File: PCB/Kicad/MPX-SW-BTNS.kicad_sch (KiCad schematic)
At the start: 34 parts, among them SW13 SWCUEL, SW14 SWPLAYL, SW15 SWRANGEL, SW16 SWSYNCL, SW17 SWLOOPL, SW18 SWSHIFTL, SW19 SWSHIFTR, SW20 SWPCUEL1, SW21 SWPCUEL2, SW22 SWCUER, SW23 SWPLAYR, SW24 SWRANGER, SW25 SWLOOPR, SW26 SWPCUEL3, SW27 SWSYNCR, SW28 SWDECKSEL, SW29 SWPADL5, SW30 SWPADL1, SW31 SWPADL6, SW32 SWPADL2, SW33 SWPADL7, SW34 SWPADL3, SW35 SWPADL4, SW36 SWPADL8, SW37 SWPADR5, SW38 SWPADR1, SW39 SWPADR6, SW40 SWPADR2, SW41 SWPADR7, SW42 SWPADR3, SW43 SWPADR4, SW44 SWPADR8

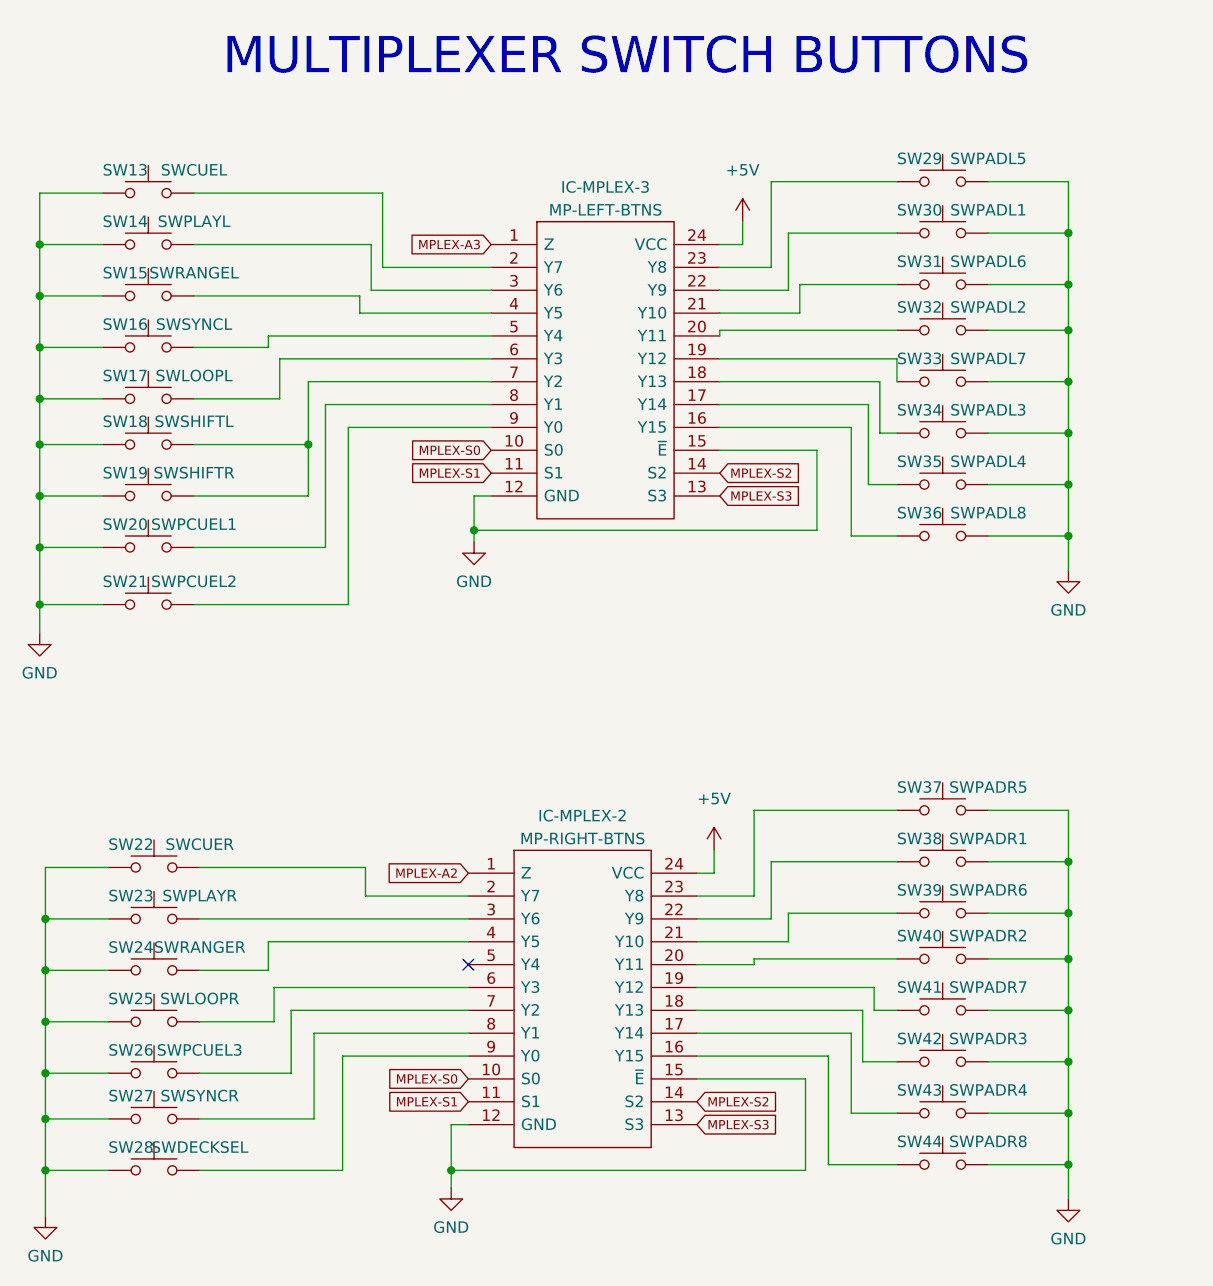
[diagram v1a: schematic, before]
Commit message: routing WIP
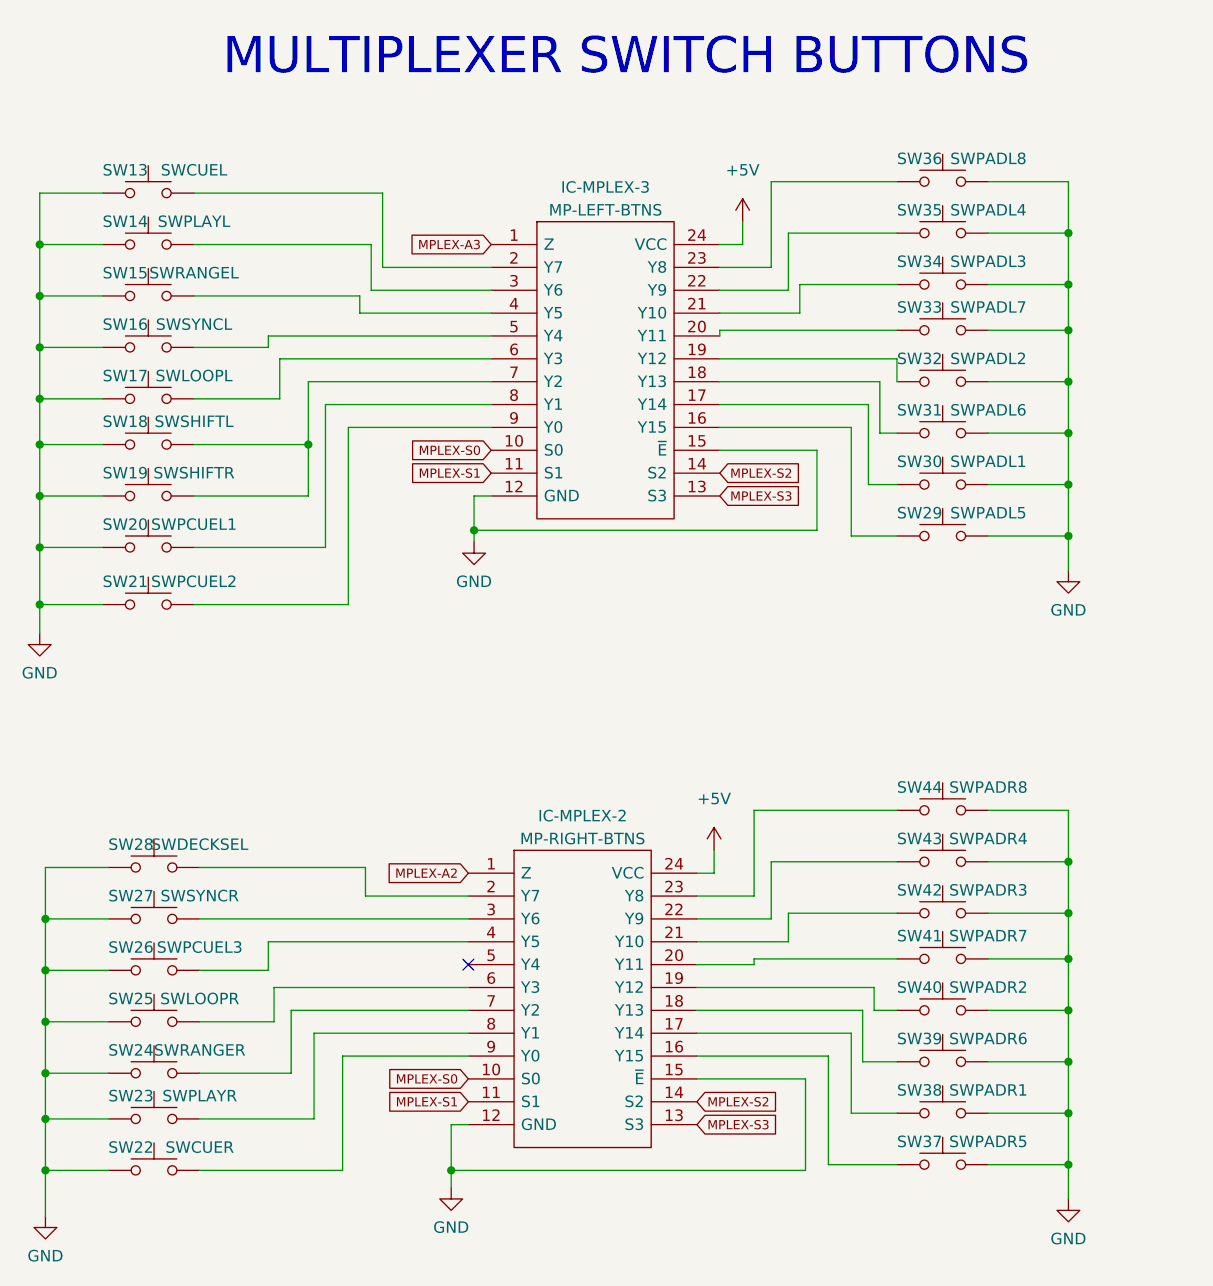
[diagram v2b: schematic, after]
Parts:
- SW13, SW14, SW15, SW16, SW17, SW18, SW19, SW20, SW21, SW22, SW23, SW24, SW25, SW26, SW27, SW28: footprint Library:SW_PUSH_6mm_H8mm -> Library:SW_Push_1P1T_NO_6x6mm_H8mm
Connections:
- net at SW41.1: now also IC-MPLEX-2.20 (Y11); no longer IC-MPLEX-2.19 (Y12)
- net at SW27.2: now also IC-MPLEX-2.3 (Y6); no longer IC-MPLEX-2.8 (Y1)
- net at IC-MPLEX-3.16 (Y15): now also SW29.1; no longer SW36.1
- net at IC-MPLEX-3.17 (Y14): now also SW30.1; no longer SW35.1
- net at IC-MPLEX-3.18 (Y13): now also SW31.1; no longer SW34.1
- net at IC-MPLEX-3.19 (Y12): now also SW32.1; no longer SW33.1
- net at IC-MPLEX-3.20 (Y11): now also SW33.1; no longer SW32.1
- net at IC-MPLEX-3.21 (Y10): now also SW34.1; no longer SW31.1
- net at IC-MPLEX-3.22 (Y9): now also SW35.1; no longer SW30.1
- net at IC-MPLEX-3.23 (Y8): now also SW36.1; no longer SW29.1
- net at SW40.1: now also IC-MPLEX-2.19 (Y12); no longer IC-MPLEX-2.20 (Y11)
- net at SW44.1: now also IC-MPLEX-2.23 (Y8); no longer IC-MPLEX-2.16 (Y15)
- net at SW38.1: now also IC-MPLEX-2.17 (Y14); no longer IC-MPLEX-2.22 (Y9)
- net at SW26.2: now also IC-MPLEX-2.4 (Y5); no longer IC-MPLEX-2.7 (Y2)
- net at SW42.1: now also IC-MPLEX-2.21 (Y10); no longer IC-MPLEX-2.18 (Y13)
- net at SW43.1: now also IC-MPLEX-2.22 (Y9); no longer IC-MPLEX-2.17 (Y14)
- net at IC-MPLEX-2.2 (Y7): now also SW28.2; no longer SW22.2
- net at SW39.1: now also IC-MPLEX-2.18 (Y13); no longer IC-MPLEX-2.21 (Y10)
- net at SW37.1: now also IC-MPLEX-2.16 (Y15); no longer IC-MPLEX-2.23 (Y8)
- net at SW23.2: now also IC-MPLEX-2.8 (Y1); no longer IC-MPLEX-2.3 (Y6)
- net at SW24.2: now also IC-MPLEX-2.7 (Y2); no longer IC-MPLEX-2.4 (Y5)
- net at IC-MPLEX-2.9 (Y0): now also SW22.2; no longer SW28.2
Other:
- moved on the sheet: SW22, SW23, SW24, SW26, SW27, SW28, SW29, SW30, SW31, SW32, SW33, SW34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
